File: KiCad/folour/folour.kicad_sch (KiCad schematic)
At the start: 34 parts, among them J1 Conn_01x02, J2 Conn_01x03, J3 Conn_01x03, J4 Conn_01x03, J5 Conn_01x03, J6 Conn_01x02, SW1 SW_Push, SW2 SW_Push, SW3 SW_Push, SW4 SW_Push, U1 74HC165, U2 74AHC595, U3 74AHC595

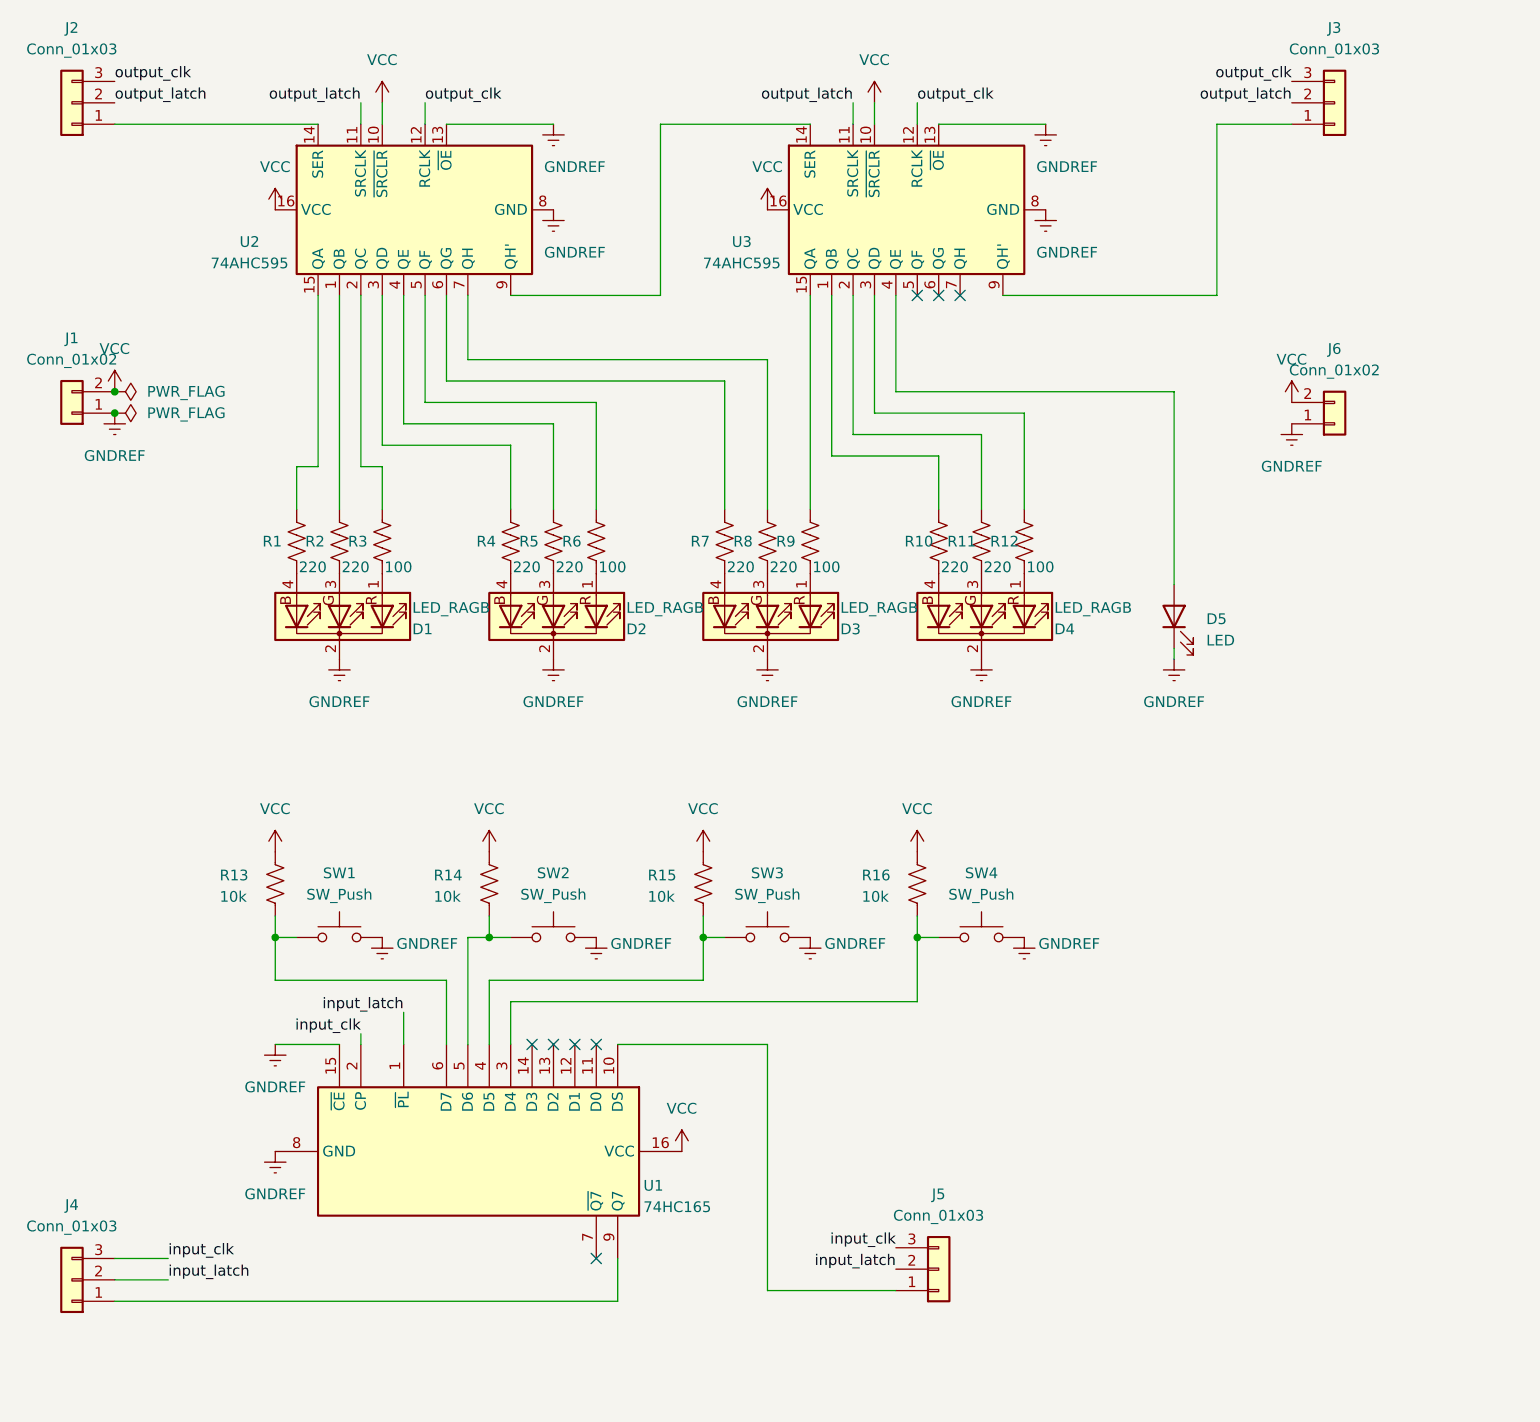
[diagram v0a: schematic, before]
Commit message: edited footprint
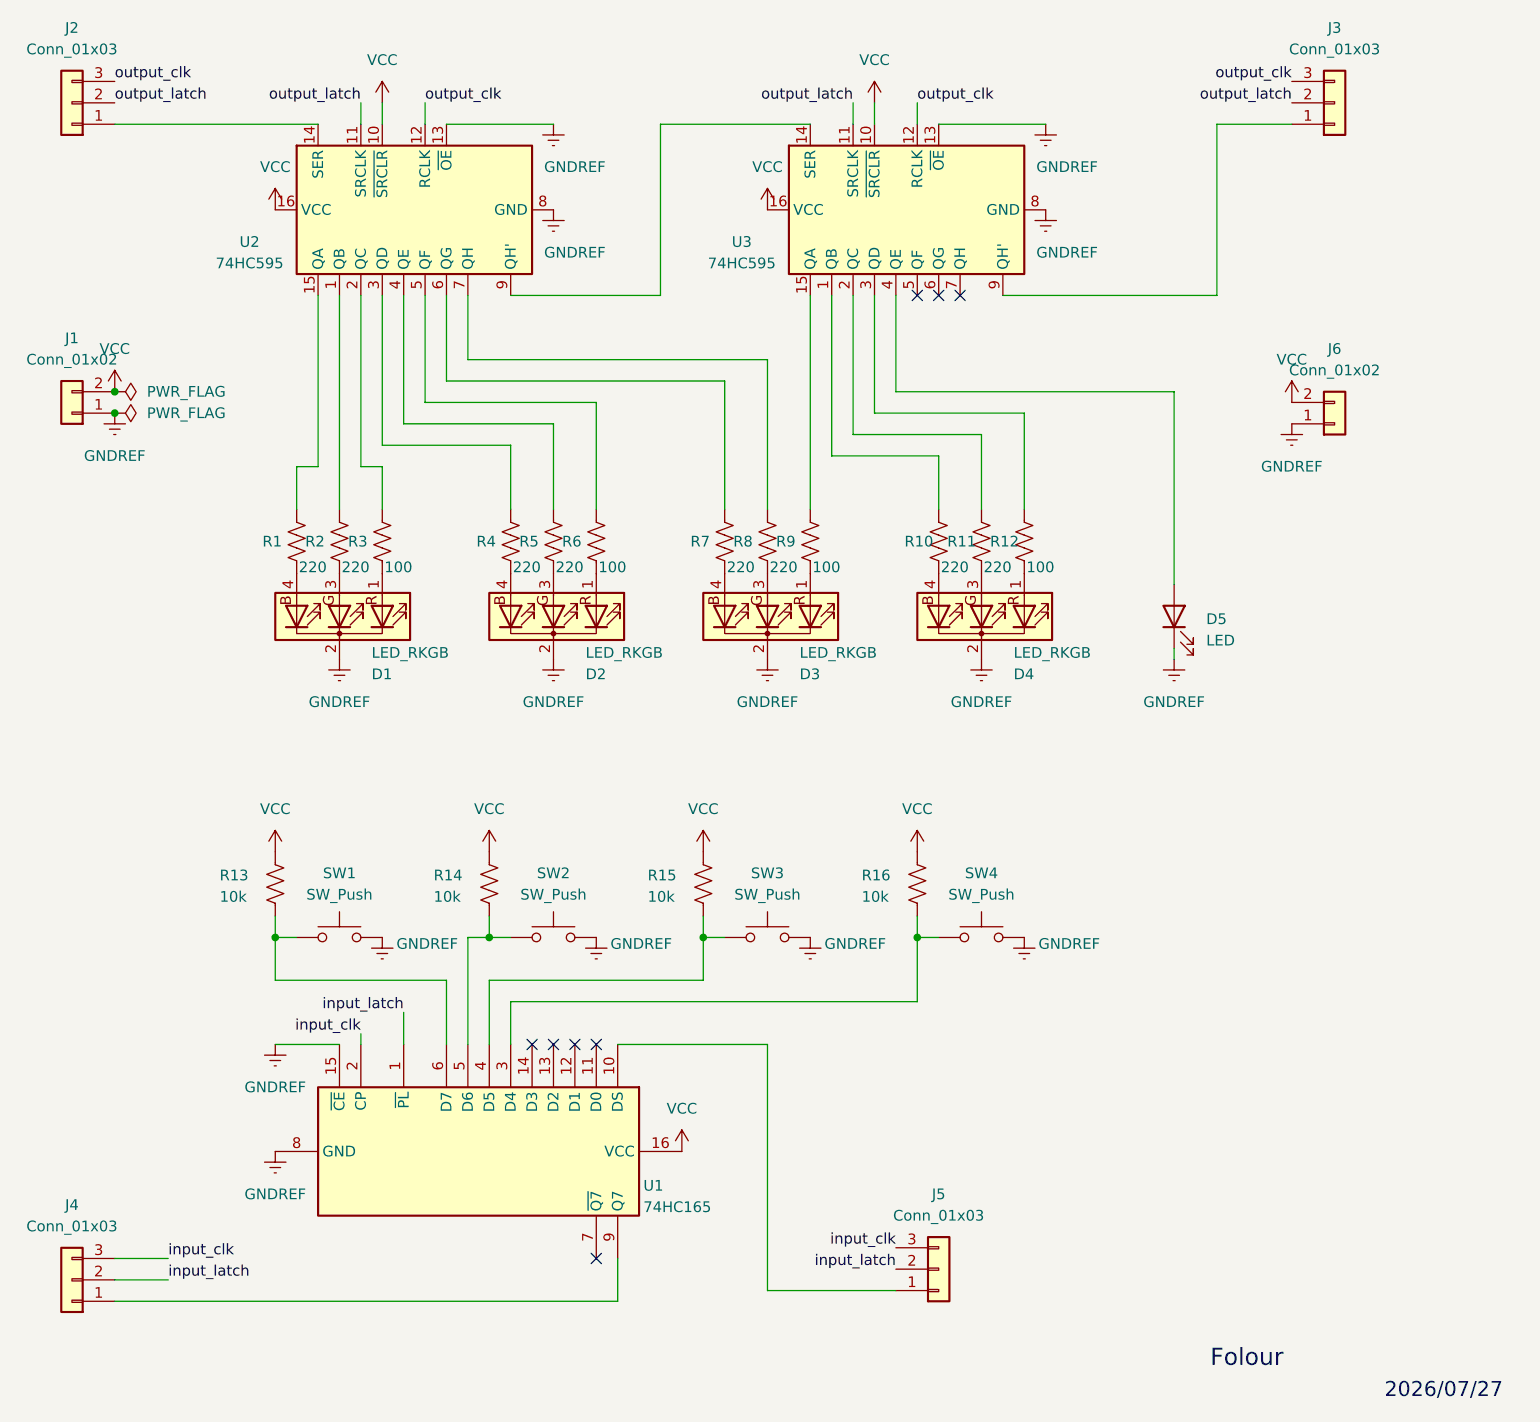
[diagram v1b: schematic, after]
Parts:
- D1, D2, D3, D4: value LED_RAGB -> LED_RKGB
- D5: footprint LED_THT:LED_D3.0mm -> LED_THT:LED_D5.0mm
- R1, R10, R11, R12, R2, R3, R4, R5, R6, R7, R8, R9: footprint Resistor_THT:R_Axial_DIN0207_L6.3mm_D2.5mm_P7.62mm_Horizontal -> Resistor_THT:R_Axial_DIN0207_L6.3mm_D2.5mm_P10.16mm_Horizontal
- R13, R14, R15, R16: footprint (none) -> Resistor_THT:R_Axial_DIN0207_L6.3mm_D2.5mm_P10.16mm_Horizontal
- SW1, SW2, SW3, SW4: footprint Button_Switch_THT:SW_PUSH_6mm -> Button_Switch_THT:SW_PUSH-12mm
- U2, U3: value 74AHC595 -> 74HC595; symbol 74xx:74AHC595 -> 74xx:74HC595
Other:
- note added: "2026/07/27"
- note added: "Folour"
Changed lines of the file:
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@@
 		)
 	)
+	(text "2026/07/27"
+		(exclude_from_sim no)
+		(at 214.884 193.548 0)
+		(effects
+			(font
+				(size 1.778 1.778)
+			)
+		)
+	)
+	(text "Folour"
+		(exclude_from_sim no)
+		(at 191.516 189.738 0)
+		(effects
+			(font
+				(size 2.032 2.032)
+			)
+		)
+	)
 	(label "output_clk"
 		(at 152.4 40.64 0)
@@
 			)
 		)
-		(property "Footprint" "Resistor_THT:R_Axial_DIN0207_L6.3mm_D2.5mm_P7.62mm_Horizontal"
+		(property "Footprint" "Resistor_THT:R_Axial_DIN0207_L6.3mm_D2.5mm_P10.16mm_Horizontal"
 			(at 105.156 92.964 90)
 			(effects
@@
 			)
 		)
-		(property "Footprint" "Resistor_THT:R_Axial_DIN0207_L6.3mm_D2.5mm_P7.62mm_Horizontal"
+		(property "Footprint" "Resistor_THT:R_Axial_DIN0207_L6.3mm_D2.5mm_P10.16mm_Horizontal"
 			(at 110.236 92.964 90)
 			(effects
@@
 			)
 		)
-		(property "Footprint" "Button_Switch_THT:SW_PUSH_6mm"
+		(property "Footprint" "Button_Switch_THT:SW_PUSH-12mm"
 			(at 160.02 134.62 0)
 			(effects
@@
 		(dnp no)
 		(property "Reference" "D4"
-			(at 168.656 103.124 90)
+			(at 163.83 108.458 90)
 			(effects
 				(font
@@
 			)
 		)
-		(property "Value" "LED_RAGB"
-			(at 168.656 100.584 90)
+		(property "Value" "LED_RKGB"
+			(at 163.83 105.918 90)
 			(effects
 				(font
@@
 			)
 		)
-		(property "Footprint" "Resistor_THT:R_Axial_DIN0207_L6.3mm_D2.5mm_P7.62mm_Horizontal"
+		(property "Footprint" "Resistor_THT:R_Axial_DIN0207_L6.3mm_D2.5mm_P10.16mm_Horizontal"
 			(at 84.836 92.964 90)
 			(effects
@@
 			)
 		)
-		(property "Footprint" "Resistor_THT:R_Axial_DIN0207_L6.3mm_D2.5mm_P7.62mm_Horizontal"
+		(property "Footprint" "Resistor_THT:R_Axial_DIN0207_L6.3mm_D2.5mm_P10.16mm_Horizontal"
 			(at 89.916 92.964 90)
 			(effects
@@
 			)
 		)
-		(property "Footprint" "Resistor_THT:R_Axial_DIN0207_L6.3mm_D2.5mm_P7.62mm_Horizontal"
+		(property "Footprint" "Resistor_THT:R_Axial_DIN0207_L6.3mm_D2.5mm_P10.16mm_Horizontal"
 			(at 135.636 92.964 90)
 			(effects
@@
 			)
 		)
-		(property "Footprint" ""
+		(property "Footprint" "Resistor_THT:R_Axial_DIN0207_L6.3mm_D2.5mm_P10.16mm_Horizontal"
 			(at 153.416 133.604 90)
 			(effects
@@
 			)
 		)
-		(property "Footprint" "Resistor_THT:R_Axial_DIN0207_L6.3mm_D2.5mm_P7.62mm_Horizontal"
+		(property "Footprint" "Resistor_THT:R_Axial_DIN0207_L6.3mm_D2.5mm_P10.16mm_Horizontal"
 			(at 155.956 92.964 90)
 			(effects
@@
 			)
 		)
-		(property "Footprint" "LED_THT:LED_D3.0mm"
+		(property "Footprint" "LED_THT:LED_D5.0mm"
 			(at 182.88 101.6 0)
 			(effects
@@
 			)
 		)
-		(property "Footprint" "Resistor_THT:R_Axial_DIN0207_L6.3mm_D2.5mm_P7.62mm_Horizontal"
+		(property "Footprint" "Resistor_THT:R_Axial_DIN0207_L6.3mm_D2.5mm_P10.16mm_Horizontal"
 			(at 115.316 92.964 90)
 			(effects
@@
 			)
 		)
-		(property "Footprint" "Button_Switch_THT:SW_PUSH_6mm"
+		(property "Footprint" "Button_Switch_THT:SW_PUSH-12mm"
 			(at 134.62 134.62 0)
 			(effects
@@
 			)
 		)
-		(property "Footprint" "Resistor_THT:R_Axial_DIN0207_L6.3mm_D2.5mm_P7.62mm_Horizontal"
+		(property "Footprint" "Resistor_THT:R_Axial_DIN0207_L6.3mm_D2.5mm_P10.16mm_Horizontal"
 			(at 79.756 92.964 90)
 			(effects
@@
 			)
 		)
-		(property "Footprint" ""
+		(property "Footprint" "Resistor_THT:R_Axial_DIN0207_L6.3mm_D2.5mm_P10.16mm_Horizontal"
 			(at 77.216 133.604 90)
 			(effects
@@
 			)
 		)
-		(property "Footprint" ""
+		(property "Footprint" "Resistor_THT:R_Axial_DIN0207_L6.3mm_D2.5mm_P10.16mm_Horizontal"
 			(at 102.616 133.604 90)
 			(effects
@@
 			)
 		)
-		(property "Footprint" ""
+		(property "Footprint" "Resistor_THT:R_Axial_DIN0207_L6.3mm_D2.5mm_P10.16mm_Horizontal"
 			(at 128.016 133.604 90)
 			(effects
@@
 	)
 	(symbol
-		(lib_id "74xx:74AHC595")
+		(lib_id "74xx:74HC595")
 		(at 91.44 53.34 90)
 		(mirror x)
@@
 			)
 		)
-		(property "Value" "74AHC595"
+		(property "Value" "74HC595"
 			(at 73.152 59.69 90)
 			(effects
@@
 			)
 		)
-		(property "Datasheet" "https://assets.nexperia.com/documents/data-sheet/74AHC_AHCT595.pdf"
+		(property "Datasheet" "http://www.ti.com/lit/ds/symlink/sn74hc595.pdf"
 			(at 91.44 53.34 0)
 			(effects
@@
 		(dnp no)
 		(property "Reference" "D1"
-			(at 92.456 103.124 90)
+			(at 87.63 108.458 90)
 			(effects
 				(font
@@
 			)
 		)
-		(property "Value" "LED_RAGB"
-			(at 92.456 100.584 90)
+		(property "Value" "LED_RKGB"
+			(at 87.63 105.918 90)
 			(effects
 				(font
@@
 		(dnp no)
 		(property "Reference" "D3"
-			(at 143.256 103.124 90)
+			(at 138.43 108.458 90)
 			(effects
 				(font
@@
 			)
 		)
-		(property "Value" "LED_RAGB"
-			(at 143.256 100.584 90)
+		(property "Value" "LED_RKGB"
+			(at 138.43 105.918 90)
 			(effects
 				(font
@@
 			)
 		)
-		(property "Footprint" "Button_Switch_THT:SW_PUSH_6mm"
+		(property "Footprint" "Button_Switch_THT:SW_PUSH-12mm"
 			(at 109.22 134.62 0)
 			(effects
@@
 			)
 		)
-		(property "Footprint" "Resistor_THT:R_Axial_DIN0207_L6.3mm_D2.5mm_P7.62mm_Horizontal"
+		(property "Footprint" "Resistor_THT:R_Axial_DIN0207_L6.3mm_D2.5mm_P10.16mm_Horizontal"
 			(at 140.716 92.964 90)
 			(effects
@@
 			)
 		)
-		(property "Footprint" "Resistor_THT:R_Axial_DIN0207_L6.3mm_D2.5mm_P7.62mm_Horizontal"
+		(property "Footprint" "Resistor_THT:R_Axial_DIN0207_L6.3mm_D2.5mm_P10.16mm_Horizontal"
 			(at 166.116 92.964 90)
 			(effects
@@
 			)
 		)
-		(property "Footprint" "Resistor_THT:R_Axial_DIN0207_L6.3mm_D2.5mm_P7.62mm_Horizontal"
+		(property "Footprint" "Resistor_THT:R_Axial_DIN0207_L6.3mm_D2.5mm_P10.16mm_Horizontal"
 			(at 161.036 92.964 90)
 			(effects
@@
 	)
 	(symbol
-		(lib_id "74xx:74AHC595")
+		(lib_id "74xx:74HC595")
 		(at 149.86 53.34 90)
 		(mirror x)
@@
 			)
 		)
-		(property "Value" "74AHC595"
+		(property "Value" "74HC595"
 			(at 131.572 59.69 90)
 			(effects
@@
 			)
 		)
-		(property "Datasheet" "https://assets.nexperia.com/documents/data-sheet/74AHC_AHCT595.pdf"
+		(property "Datasheet" "http://www.ti.com/lit/ds/symlink/sn74hc595.pdf"
 			(at 149.86 53.34 0)
 			(effects
@@
 		(dnp no)
 		(property "Reference" "D2"
-			(at 117.856 103.124 90)
+			(at 113.03 108.458 90)
 			(effects
 				(font
@@
 			)
 		)
-		(property "Value" "LED_RAGB"
-			(at 117.856 100.584 90)
+		(property "Value" "LED_RKGB"
+			(at 113.03 105.918 90)
 			(effects
 				(font
@@
 			)
 		)
-		(property "Footprint" "Button_Switch_THT:SW_PUSH_6mm"
+		(property "Footprint" "Button_Switch_THT:SW_PUSH-12mm"
 			(at 83.82 134.62 0)
 			(effects
@@
 			)
 		)
-		(property "Footprint" "Resistor_THT:R_Axial_DIN0207_L6.3mm_D2.5mm_P7.62mm_Horizontal"
+		(property "Footprint" "Resistor_THT:R_Axial_DIN0207_L6.3mm_D2.5mm_P10.16mm_Horizontal"
 			(at 130.556 92.964 90)
 			(effects

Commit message: fixed footprints
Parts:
- J1, J6: footprint Connector_PinHeader_1.00mm:PinHeader_1x02_P1.00mm_Horizontal -> Connector_PinHeader_2.54mm:PinHeader_1x02_P2.54mm_Horizontal
- J2, J3, J4, J5: footprint Connector_PinHeader_1.00mm:PinHeader_1x03_P1.00mm_Horizontal -> Connector_PinHeader_2.54mm:PinHeader_1x03_P2.54mm_Horizontal
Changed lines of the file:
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@@
 			)
 		)
-		(property "Footprint" "Connector_PinHeader_1.00mm:PinHeader_1x03_P1.00mm_Horizontal"
+		(property "Footprint" "Connector_PinHeader_2.54mm:PinHeader_1x03_P2.54mm_Horizontal"
 			(at 201.93 40.64 0)
 			(effects
@@
 			)
 		)
-		(property "Footprint" "Connector_PinHeader_1.00mm:PinHeader_1x03_P1.00mm_Horizontal"
+		(property "Footprint" "Connector_PinHeader_2.54mm:PinHeader_1x03_P2.54mm_Horizontal"
 			(at 52.07 40.64 0)
 			(effects
@@
 			)
 		)
-		(property "Footprint" "Connector_PinHeader_1.00mm:PinHeader_1x02_P1.00mm_Horizontal"
+		(property "Footprint" "Connector_PinHeader_2.54mm:PinHeader_1x02_P2.54mm_Horizontal"
 			(at 201.93 78.74 0)
 			(effects
@@
 			)
 		)
-		(property "Footprint" "Connector_PinHeader_1.00mm:PinHeader_1x02_P1.00mm_Horizontal"
+		(property "Footprint" "Connector_PinHeader_2.54mm:PinHeader_1x02_P2.54mm_Horizontal"
 			(at 52.07 77.47 0)
 			(effects
@@
 			)
 		)
-		(property "Footprint" "Connector_PinHeader_1.00mm:PinHeader_1x03_P1.00mm_Horizontal"
+		(property "Footprint" "Connector_PinHeader_2.54mm:PinHeader_1x03_P2.54mm_Horizontal"
 			(at 154.94 179.07 0)
 			(effects
@@
 			)
 		)
-		(property "Footprint" "Connector_PinHeader_1.00mm:PinHeader_1x03_P1.00mm_Horizontal"
+		(property "Footprint" "Connector_PinHeader_2.54mm:PinHeader_1x03_P2.54mm_Horizontal"
 			(at 52.07 180.34 0)
 			(effects
